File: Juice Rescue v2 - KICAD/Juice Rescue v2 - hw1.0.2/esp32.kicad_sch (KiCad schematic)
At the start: 43 parts, among them J2 USB_C_Receptacle_USB2.0_16P, J3 Conn_01x06, Q3 BSS138, Q4 BSS138, Q5 AO3400A, Q6 MMBT3904, Q7 MMBT3904, U3 MCP9808_MSOP, U5 ESP32-S3-WROOM-2, U6 USBLC6-2SC6

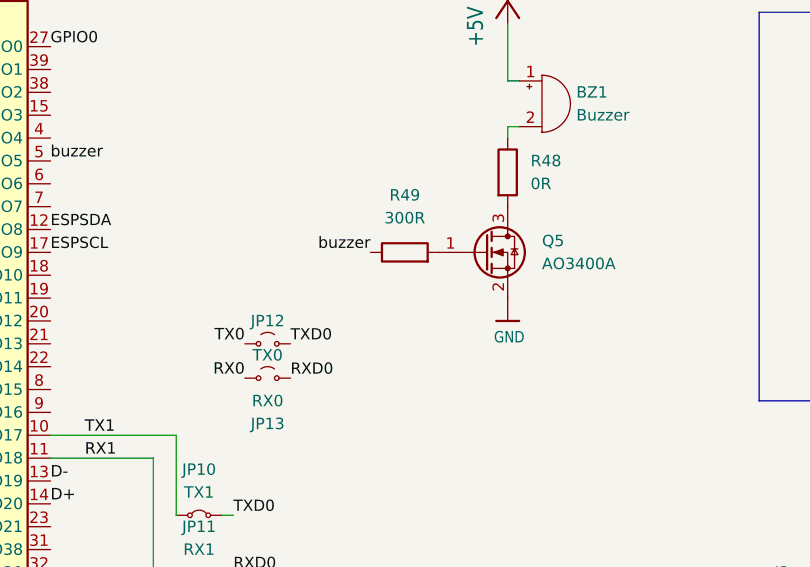
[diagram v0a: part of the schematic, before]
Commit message: Hw changes.
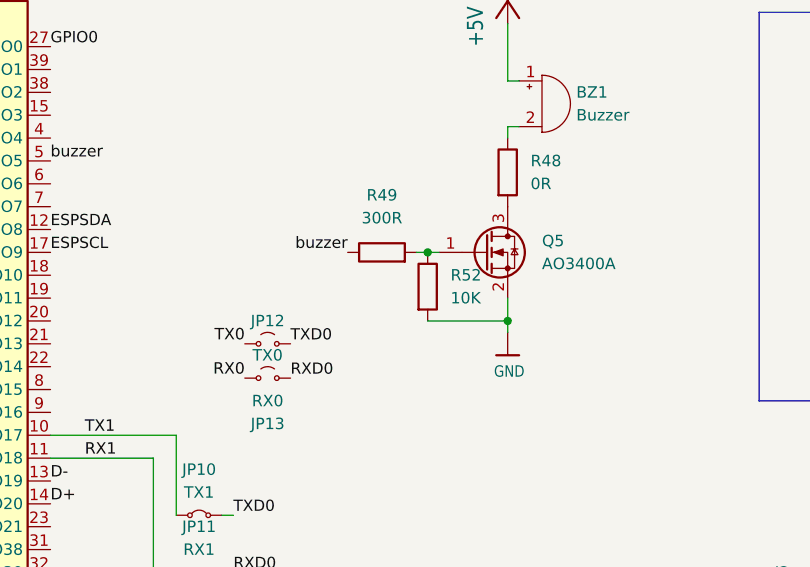
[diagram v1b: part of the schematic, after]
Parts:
- added R52: 10K, symbol Device:R
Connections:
- net GND: now also R52.2
- net at Q5.1 (G), R49.2: now also R52.1
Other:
- moved on the sheet: R49
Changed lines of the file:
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@@
 	)
 	(junction
+		(at 104.14 113.03)
+		(diameter 0)
+		(color 0 0 0 0)
+	)
+	(junction
 		(at 214.63 68.58)
 		(diameter 0)
@@
 	)
 	(junction
+		(at 95.25 105.41)
+		(diameter 0)
+		(color 0 0 0 0)
+	)
+	(junction
 		(at 149.86 148.59)
 		(diameter 0)
@@
 	(wire
 		(pts
+			(xy 95.25 113.03) (xy 104.14 113.03)
+		)
+		(stroke
+			(width 0)
+			(type default)
+		)
+	)
+	(wire
+		(pts
 			(xy 182.88 133.35) (xy 172.72 133.35)
 		)
@@
 	(wire
 		(pts
+			(xy 104.14 113.03) (xy 104.14 110.49)
+		)
+		(stroke
+			(width 0)
+			(type default)
+		)
+	)
+	(wire
+		(pts
 			(xy 156.21 163.83) (xy 152.4 163.83)
 		)
@@
 	(wire
 		(pts
+			(xy 104.14 114.3) (xy 104.14 113.03)
+		)
+		(stroke
+			(width 0)
+			(type default)
+		)
+	)
+	(wire
+		(pts
 			(xy 212.09 68.58) (xy 207.01 68.58)
 		)
@@
 	(wire
 		(pts
+			(xy 95.25 105.41) (xy 96.52 105.41)
+		)
+		(stroke
+			(width 0)
+			(type default)
+		)
+	)
+	(wire
+		(pts
 			(xy 69.85 41.91) (xy 69.85 44.45)
 		)
@@
 	(wire
 		(pts
+			(xy 93.98 105.41) (xy 95.25 105.41)
+		)
+		(stroke
+			(width 0)
+			(type default)
+		)
+	)
+	(wire
+		(pts
 			(xy 53.34 128.27) (xy 64.77 128.27)
 		)
@@
 	)
 	(label "buzzer"
-		(at 88.9 105.41 180)
+		(at 86.36 105.41 180)
 		(effects
 			(font
@@
 	(symbol
 		(lib_id "Juice Rescue v2 - hw1.0.2-eagle-import:microbuilder_GND")
-		(at 104.14 113.03 0)
+		(at 104.14 116.84 0)
 		(unit 1)
 		(exclude_from_sim no)
@@
 		(dnp no)
 		(property "Reference" "#U$030"
-			(at 104.14 113.03 0)
+			(at 104.14 116.84 0)
 			(effects
 				(font
@@
 		)
 		(property "Value" "GND"
-			(at 102.616 115.57 0)
+			(at 102.616 119.38 0)
 			(effects
 				(font
@@
 		)
 		(property "Footprint" ""
-			(at 104.14 113.03 0)
+			(at 104.14 116.84 0)
 			(effects
 				(font
@@
 		)
 		(property "Datasheet" ""
-			(at 104.14 113.03 0)
+			(at 104.14 116.84 0)
 			(effects
 				(font
@@
 		)
 		(property "Description" ""
-			(at 104.14 113.03 0)
+			(at 104.14 116.84 0)
 			(effects
 				(font
@@
 	(symbol
 		(lib_id "Device:R")
-		(at 92.71 105.41 90)
+		(at 90.17 105.41 90)
 		(unit 1)
 		(exclude_from_sim no)
@@
 		(fields_autoplaced yes)
 		(property "Reference" "R49"
-			(at 92.71 99.06 90)
+			(at 90.17 99.06 90)
 			(effects
 				(font
@@
 		)
 		(property "Value" "300R"
-			(at 92.71 101.6 90)
+			(at 90.17 101.6 90)
 			(effects
 				(font
@@
 		)
 		(property "Footprint" "PCM_JLCPCB:R_0603"
-			(at 92.71 107.188 90)
+			(at 90.17 107.188 90)
 			(effects
 				(font
@@
 		)
 		(property "Datasheet" "~"
-			(at 92.71 105.41 0)
+			(at 90.17 105.41 0)
 			(effects
 				(font
@@
 		)
 		(property "Description" "Resistor"
-			(at 92.71 105.41 0)
+			(at 90.17 105.41 0)
 			(effects
 				(font
@@
 					(unit 1)
 				)
+			)
+		)
+	)
+	(symbol
+		(lib_id "Device:R")
+		(at 95.25 109.22 0)
+		(unit 1)
+		(exclude_from_sim no)
+		(in_bom yes)
+		(on_board yes)
+		(dnp no)
+		(fields_autoplaced yes)
+		(property "Reference" "R52"
+			(at 97.79 107.9499 0)
+			(effects
+				(font
+					(size 1.27 1.27)
+				)
+				(justify left)
+			)
+		)
+		(property "Value" "10K"
+			(at 97.79 110.4899 0)
+			(effects
+				(font
+					(size 1.27 1.27)
+				)
+				(justify left)
+			)
+		)
+		(property "Footprint" ""
+			(at 93.472 109.22 90)
+			(effects
+				(font
+					(size 1.27 1.27)
+				)
+				(hide yes)
+			)
+		)
+		(property "Datasheet" "~"
+			(at 95.25 109.22 0)
+			(effects
+				(font
+					(size 1.27 1.27)
+				)
+				(hide yes)
+			)
+		)
+		(property "Description" "Resistor"
+			(at 95.25 109.22 0)
+			(effects
+				(font
+					(size 1.27 1.27)
+				)
+				(hide yes)
+			)
+		)
+		(pin "2"
+		)
+		(pin "1"
+		)
+		(instances
+			(project ""
+				(path "/dc23f6cf-65e9-4621-9791-f98f2f73fe59/9fe9eeef-2b06-4079-8ab9-e76c0634f520"
+					(reference "R52")
+					(unit 1)
+				)
